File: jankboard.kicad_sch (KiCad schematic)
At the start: 154 parts, among them J1 F31L-1A7H1-11030, J2 F31L-1A7H1-11030, J3 Conn_01x02, J4 Conn_01x02, SW1 SW_Push_45deg, SW10 SW_Push_45deg, SW11 SW_Push_45deg, SW12 SW_Push_45deg, SW13 SW_Push_45deg, SW14 SW_Push_45deg, SW15 SW_Push_45deg, SW16 SW_Push_45deg, SW17 SW_Push_45deg, SW18 SW_Push_45deg, SW19 SW_Push_45deg, SW2 SW_Push_45deg, SW20 SW_Push_45deg, SW21 SW_Push_45deg, SW3 SW_Push_45deg, SW4 SW_Push_45deg, SW5 SW_Push_45deg, SW6 SW_Push_45deg, SW7 SW_Push_45deg, SW8 SW_Push_45deg, SW9 SW_Push_45deg, U1 nice_nano

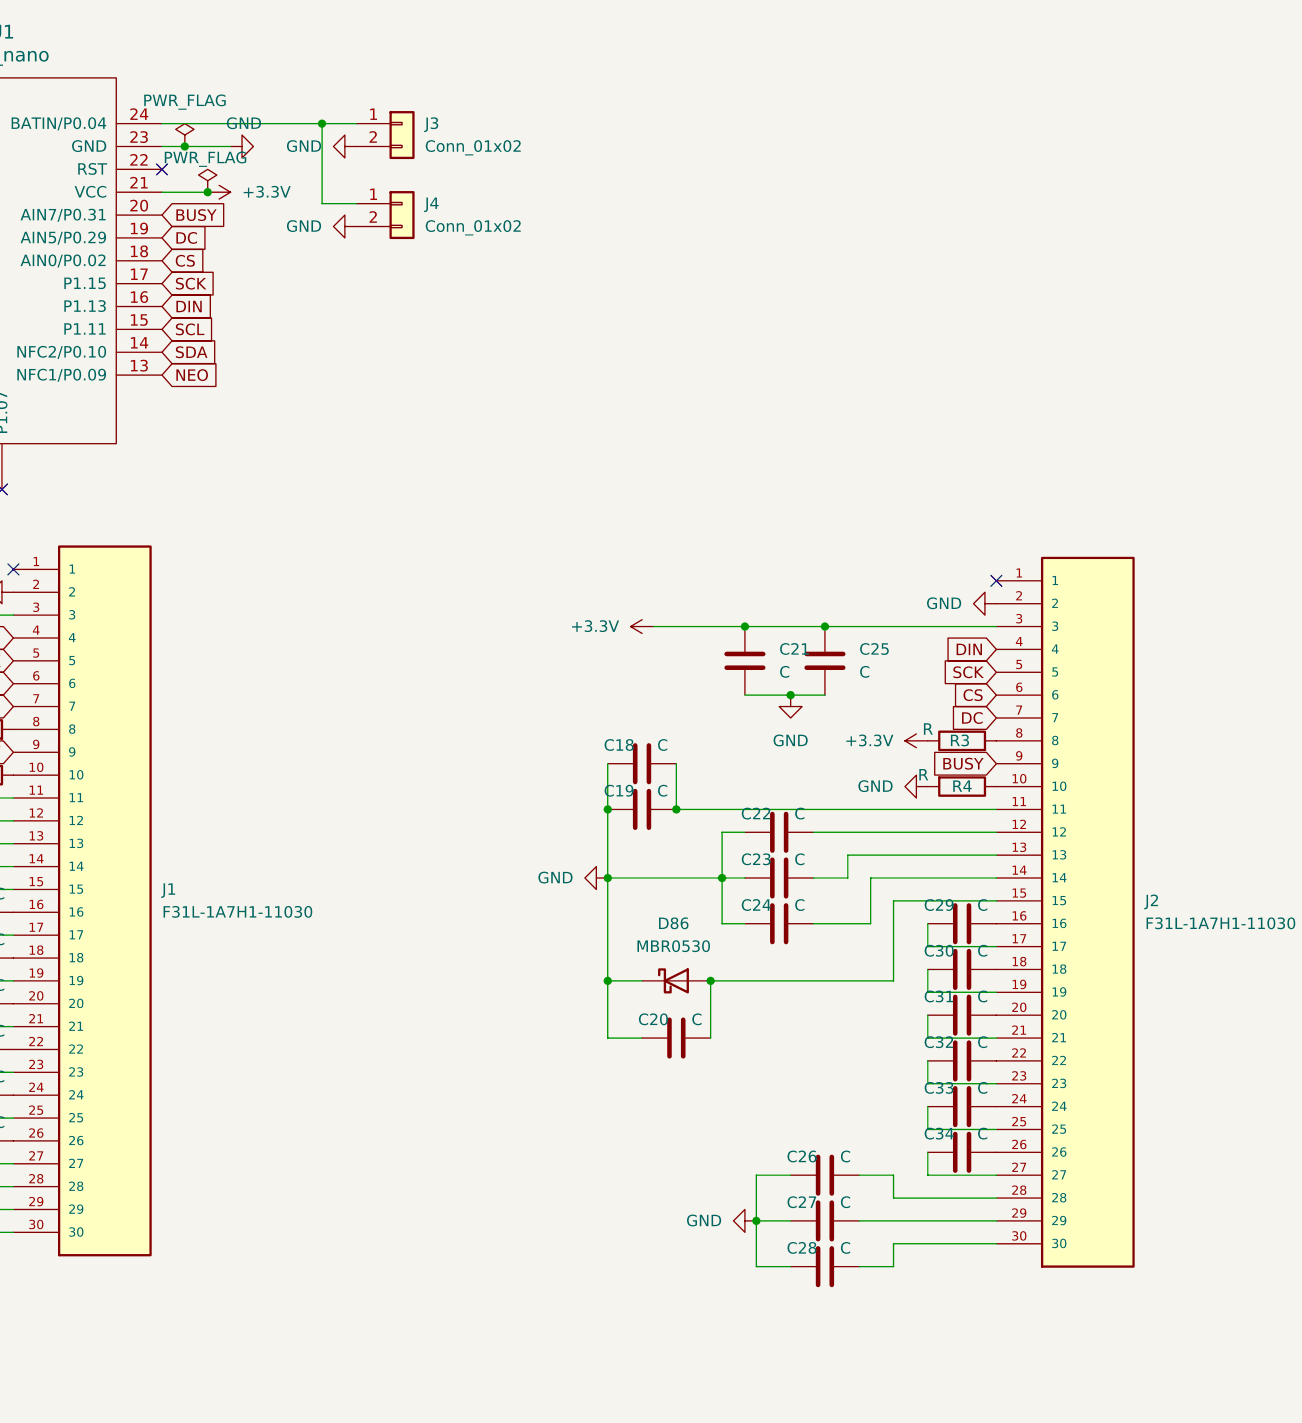
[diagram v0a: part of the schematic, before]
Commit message: connectors
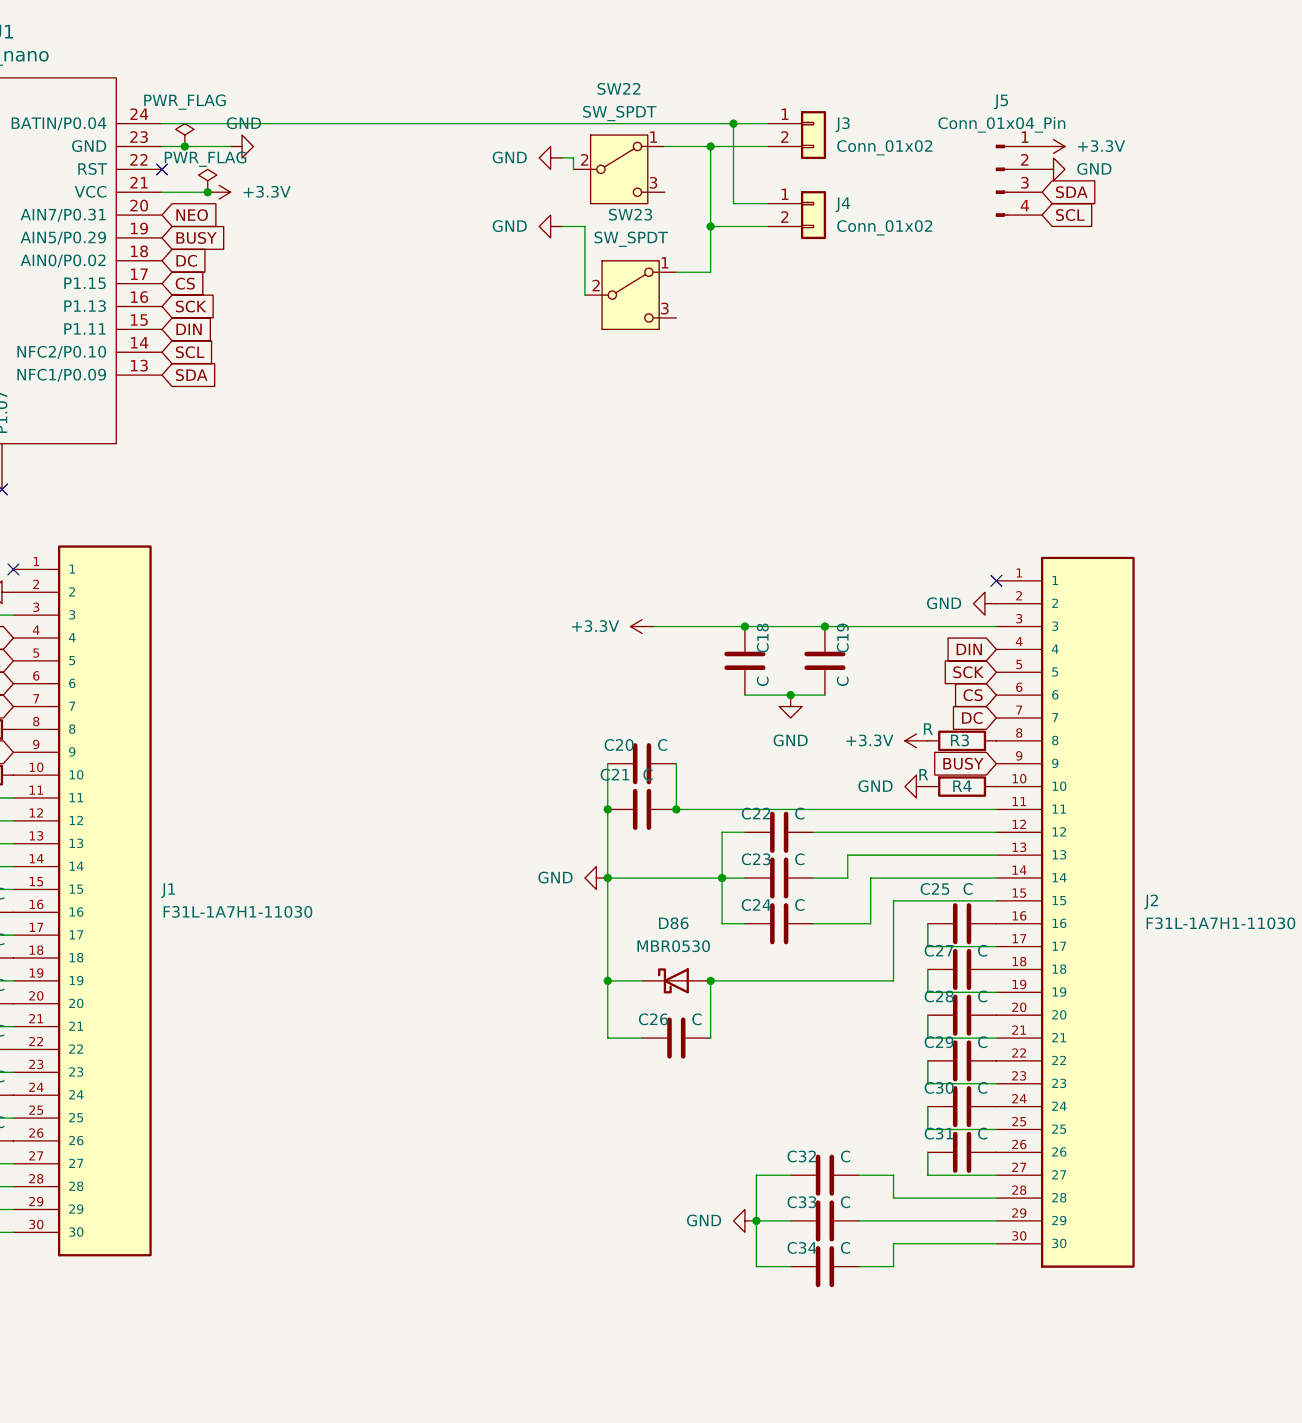
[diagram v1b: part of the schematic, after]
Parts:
- added J5: Conn_01x04_Pin, symbol Connector:Conn_01x04_Pin
- added SW22, SW23: SW_SPDT, symbol Switch:SW_SPDT
- J3, J4: footprint Connector_JST:JST_EH_S2B-EH_1x02_P2.50mm_Horizontal -> Connector_JST:JST_PH_S2B-PH-SM4-TB_1x02-1MP_P2.00mm_Horizontal
- R1, R2, R3, R4, R5, R6, R7, R8: footprint Resistor_SMD:R_0612_1632Metric -> Resistor_SMD:R_0603_1608Metric
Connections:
- net +3.3V: now also C18.1, C19.1, J5.1 (Pin_1); no longer C21.1, C25.1
- net BUSY: now also U1.19 (AIN5/P0.29); no longer U1.20 (AIN7/P0.31)
- net CS: now also U1.17 (P1.15); no longer U1.18 (AIN0/P0.02)
- net DC: now also U1.18 (AIN0/P0.02); no longer U1.19 (AIN5/P0.29)
- net DIN: now also U1.15 (P1.11); no longer U1.16 (P1.13)
- net GND: now also C18.2, C19.2, C21.1, C32.1, C33.1, C34.1, J5.2 (Pin_2), SW22.2 (B), SW23.2 (B); no longer C18.1, C19.1, C21.2, C25.2, C27.1, C28.1, J3.2 (Pin_2), J4.2 (Pin_2)
- net NEO: now also U1.20 (AIN7/P0.31); no longer U1.13 (NFC1/P0.09)
- net SCK: now also U1.16 (P1.13); no longer U1.17 (P1.15)
- net SCL: now also U1.14 (NFC2/P0.10), J5.4 (Pin_4); no longer U1.15 (P1.11)
- net SDA: now also U1.13 (NFC1/P0.09), J5.3 (Pin_3); no longer U1.14 (NFC2/P0.10)
- net at C26.2: now also D86.2 (A), J2.15; no longer J2.28
- net at C27.2: now also J2.18; no longer J2.29
- net at C29.1: now also J2.23; no longer J2.17
- net at C29.2: now also J2.22; no longer J2.16
- net at C28.2: now also J2.20; no longer J2.30
- net at J2.27: now also C31.1; no longer C34.1
- net at C34.2: now also J2.30; no longer J2.26
- net at C30.2: now also J2.24; no longer J2.18
- net at J2.19: now also C27.1; no longer C30.1
- net at C31.2: now also J2.26; no longer J2.20
- net at J2.21: now also C28.1; no longer C31.1
- net at C32.2: now also J2.28; no longer J2.22
- net at C33.2: now also J2.29; no longer J2.24
- net at J2.25: now also C30.1; no longer C33.1
- new net: C20.2, C21.2, J2.11
- new net: J3.2 (Pin_2), J4.2 (Pin_2), SW22.1 (A), SW23.1 (A)
- new net: C25.2, J2.16
- new net: C25.1, J2.17
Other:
- moved on the sheet: C18, C19, C20, C21, C25, C26, C27, C28, C29, C30, C31, C32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
